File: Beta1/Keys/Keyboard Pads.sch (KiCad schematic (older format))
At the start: 46 parts, among them U1 MPR121TH, U2 MPR121TH, U3 MPR121TH

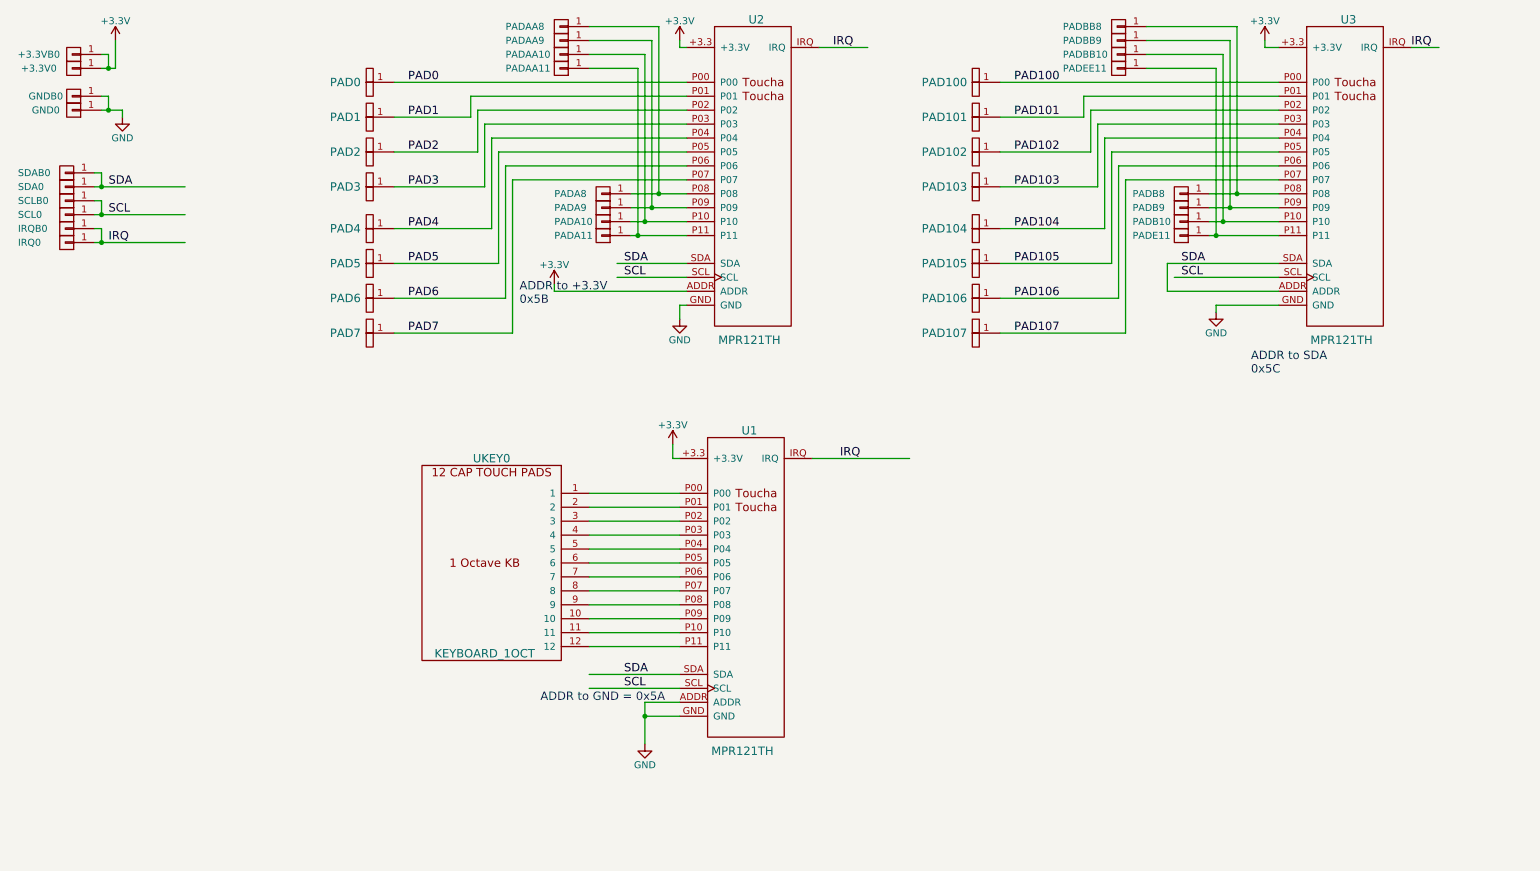
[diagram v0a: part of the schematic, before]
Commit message: Minor Fuss. Apologies.
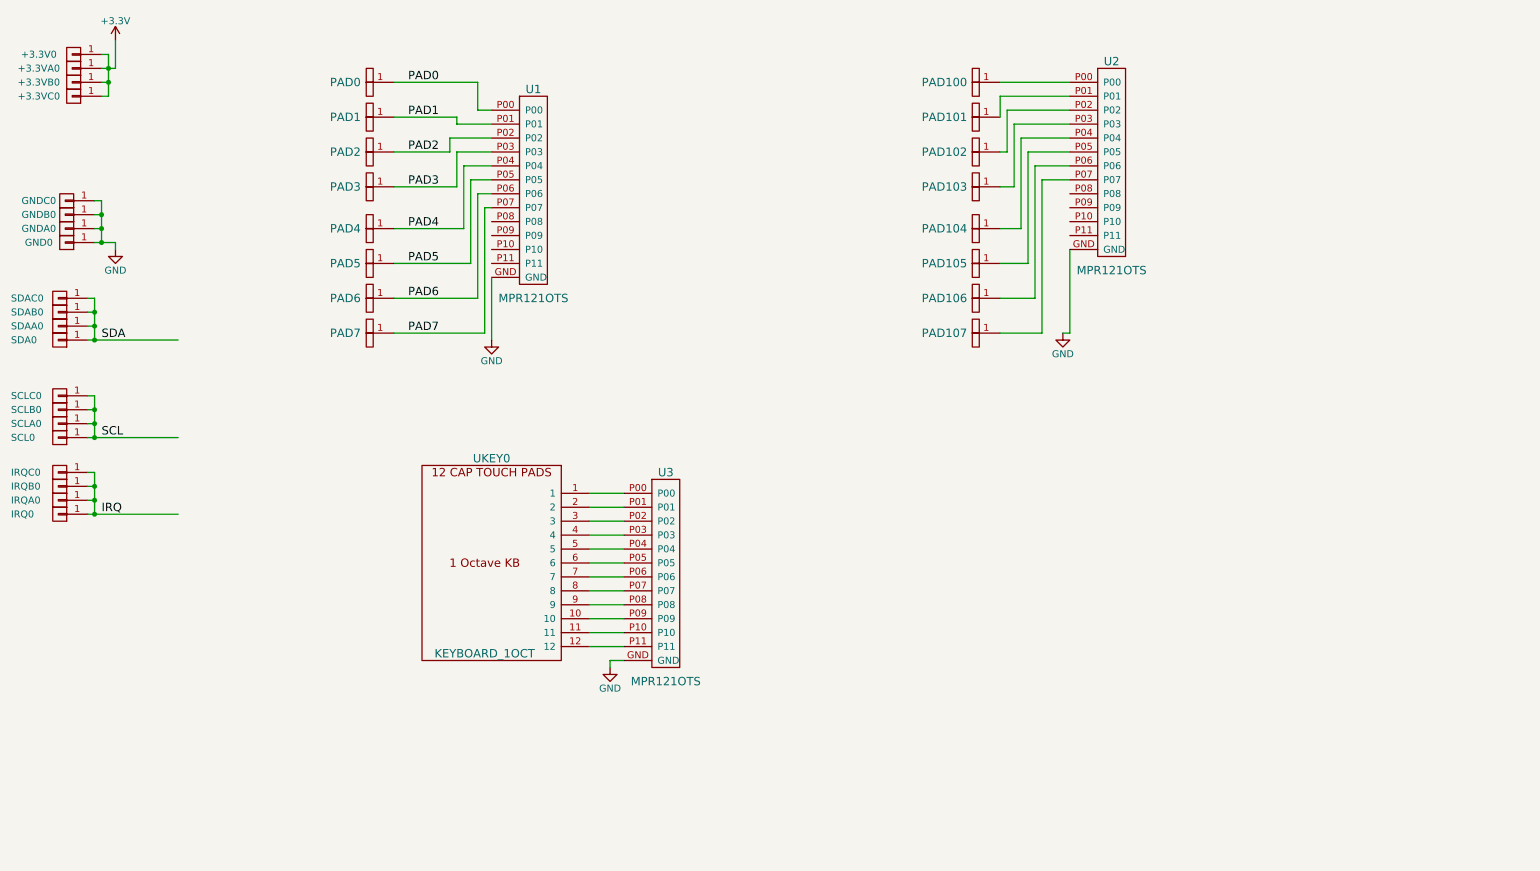
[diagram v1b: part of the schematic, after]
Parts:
- removed PADA10, PADA11, PADA8, PADA9, PADAA10, PADAA11, PADAA8, PADAA9, PADB10, PADB8, PADB9, PADBB10, PADBB8, PADBB9, PADE11, PADEE11: CONN_01X01, Liberry:single_0.1, symbol CONN_01X01
- removed U1, U2, U3: MPR121TH, Liberry:MPR121TH, symbol MPR121TH
- added +3.3VB0, +3.3VC0, GNDB0, GNDC0, IRQB0, IRQC0, SCLB0, SCLC0, SDAB0, SDAC0: CONN_01X01, Liberry:single_0.1, symbol CONN_01X01
- added U1, U2, U3: MPR121OTS, Liberry:MPR121OTS, symbol MPR121OTS
- renumbered +3.3VB0 to +3.3V0, +3.3V0 to +3.3VA0, GNDB0 to GNDA0, IRQB0 to IRQA0, SCLB0 to SCLA0, SDAB0 to SDAA0
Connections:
- net labels removed: PAD100, PAD101, PAD102, PAD103, PAD104, PAD105, PAD106, PAD107
- wire segments 123 -> 89
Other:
- note removed: "ADDR to +3.3V\n0x5B\n"
- note removed: "ADDR to GND = 0x5A"
- note removed: "ADDR to SDA\n0x5C"
- moved on the sheet: GND0, GNDA0, IRQ0, IRQA0, SCL0, SCLA0, SDA0, SDAA0
